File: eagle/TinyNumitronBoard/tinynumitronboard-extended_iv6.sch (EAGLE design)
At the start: 33 parts

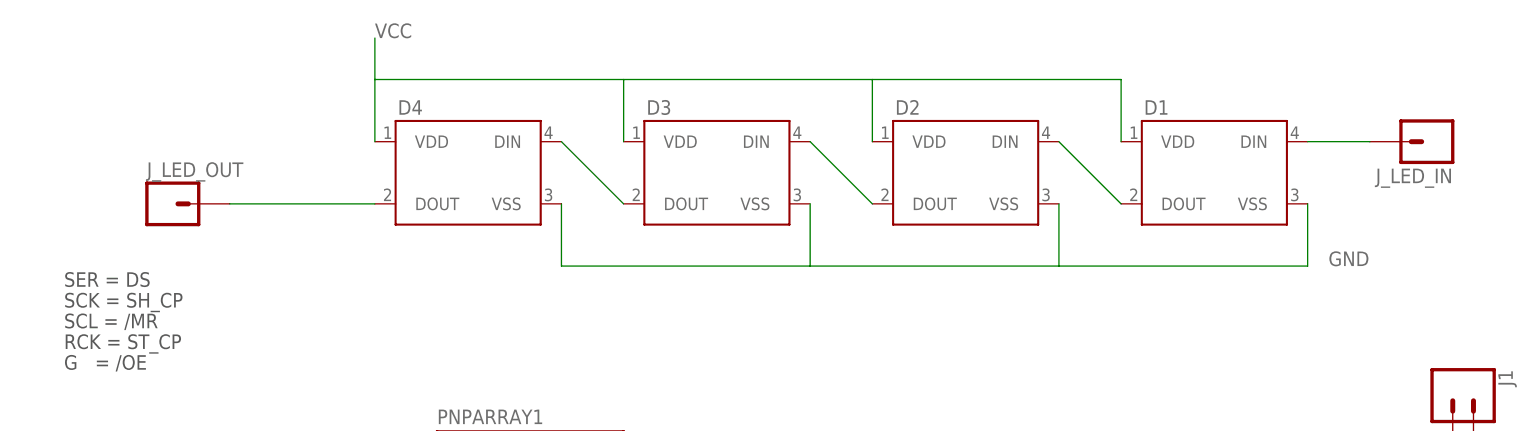
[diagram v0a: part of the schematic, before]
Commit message: Final commit before sending v2.0 to production
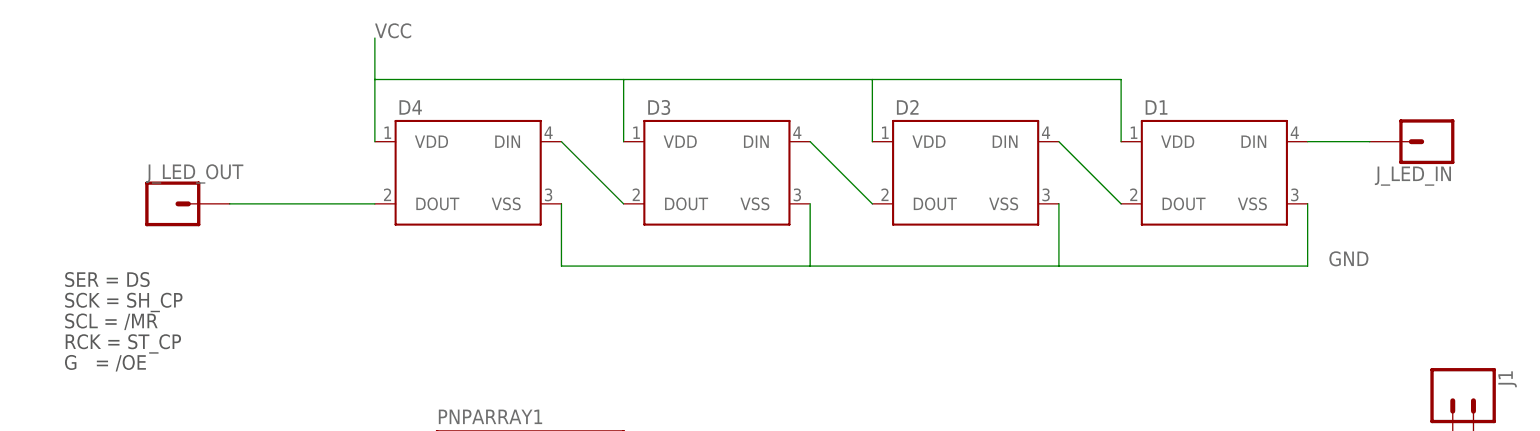
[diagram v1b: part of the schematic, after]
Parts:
- J_LED_IN, J_LED_OUT: device SparkFun-Connectors:M01NOSILK-KIT -> SparkFun-Connectors:CONN_01
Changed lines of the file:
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@@
 <part name="D3" library="SparkFun-LED" deviceset="WS2812B" device=""/>
 <part name="D4" library="SparkFun-LED" deviceset="WS2812B" device=""/>
-<part name="J_LED_IN" library="SparkFun-Connectors" deviceset="M01" device="NOSILK-KIT"/>
-<part name="J_LED_OUT" library="SparkFun-Connectors" deviceset="M01" device="NOSILK-KIT"/>
+<part name="J_LED_IN" library="SparkFun-Connectors" deviceset="CONN_01" device=""/>
+<part name="J_LED_OUT" library="SparkFun-Connectors" deviceset="CONN_01" device=""/>
 <part name="TUBE2" library="kalshagar" deviceset="IV6_NUMITRON" device="LARGE" value="IV6_NUMITRONLARGE"/>
 <part name="SER2" library="SparkFun-DigitalIC" deviceset="74*595" device="D" technology="LS"/>
